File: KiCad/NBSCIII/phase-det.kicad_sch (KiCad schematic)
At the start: 34 parts, among them Q1100 BC337-25, U1 LM324N

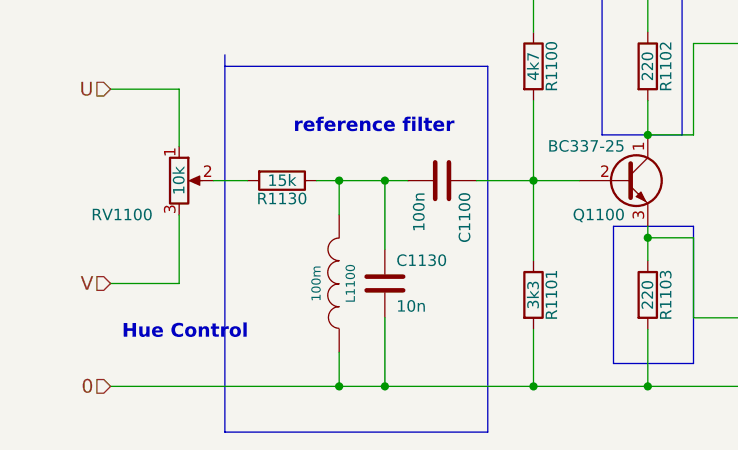
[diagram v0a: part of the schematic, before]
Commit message: unrescue Device:L_small
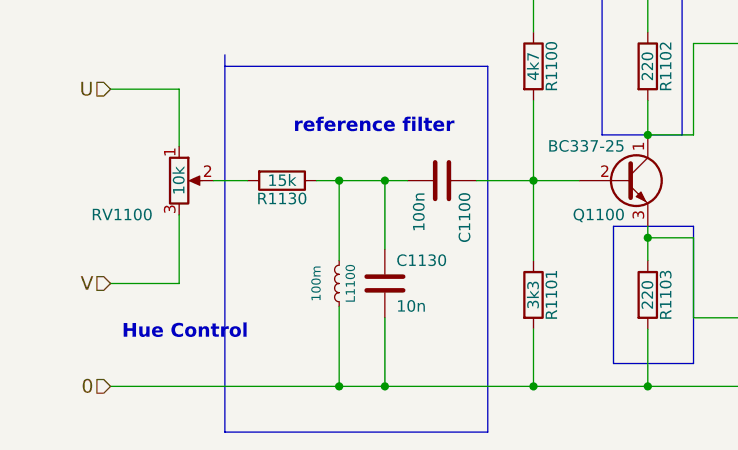
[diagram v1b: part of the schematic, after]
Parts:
- L1100: symbol NBSCIII-rescue:INDUCTOR -> Device:L_Small
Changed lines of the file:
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@@
     (stroke (width 0) (type default) (color 0 0 0 0))
   )
-  (wire (pts (xy 50.8 66.04) (xy 50.8 69.85))
+  (wire (pts (xy 50.8 60.96) (xy 50.8 69.85))
     (stroke (width 0) (type default) (color 0 0 0 0))
   )
@@
     (stroke (width 0) (type default) (color 0 0 0 0))
   )
-  (wire (pts (xy 50.8 50.8) (xy 50.8 46.99))
+  (wire (pts (xy 50.8 46.99) (xy 50.8 55.88))
     (stroke (width 0) (type default) (color 0 0 0 0))
   )
@@
     (pin "3")
   )
-  (symbol (lib_id "NBSCIII-rescue:INDUCTOR") (at 50.8 58.42 180) (unit 1)
+  (symbol (lib_id "Device:L_Small") (at 50.8 58.42 180) (unit 1)
     (in_bom yes) (on_board yes)
     (property "Reference" "L1100" (id 0) (at 52.07 58.42 90)
